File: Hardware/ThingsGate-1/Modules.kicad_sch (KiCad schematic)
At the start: 5 parts, among them SW1 DSHP03TS-S, U1 CH334R, U2 ThingsCore-1, U7 mPCIE-52P-SLOT, U8 mPCIE-52P-SLOT

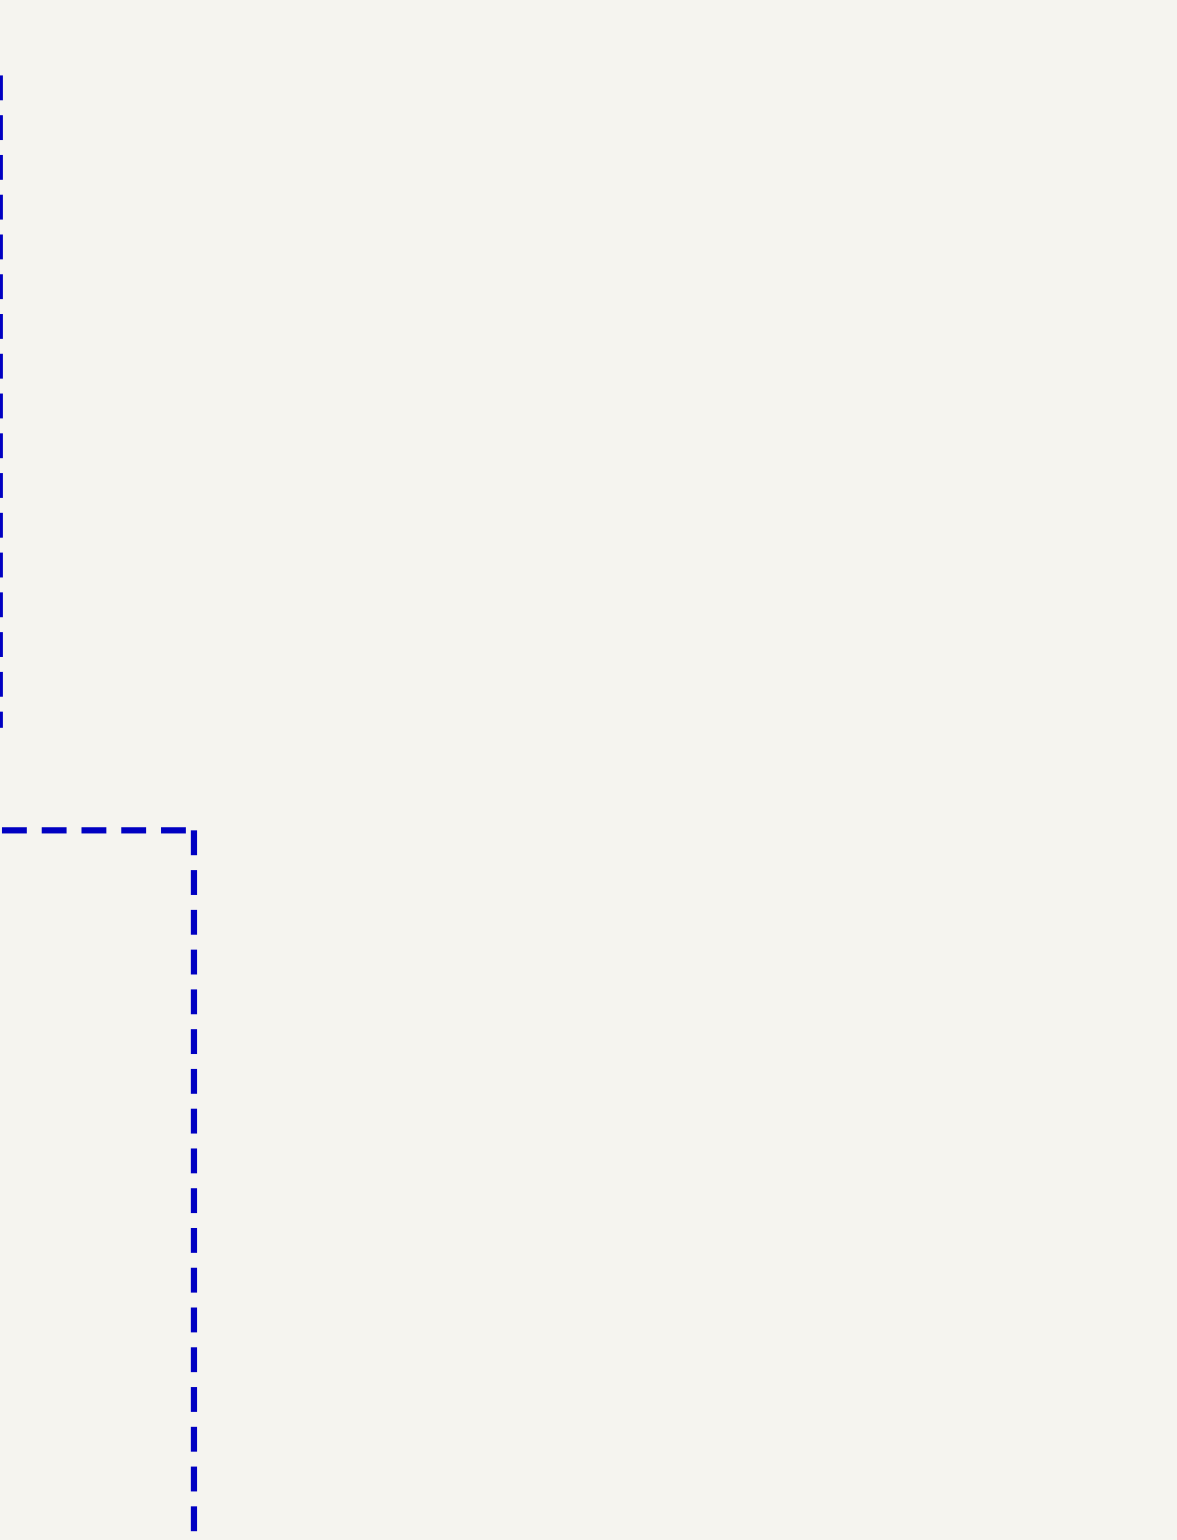
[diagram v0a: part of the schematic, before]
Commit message: schematic
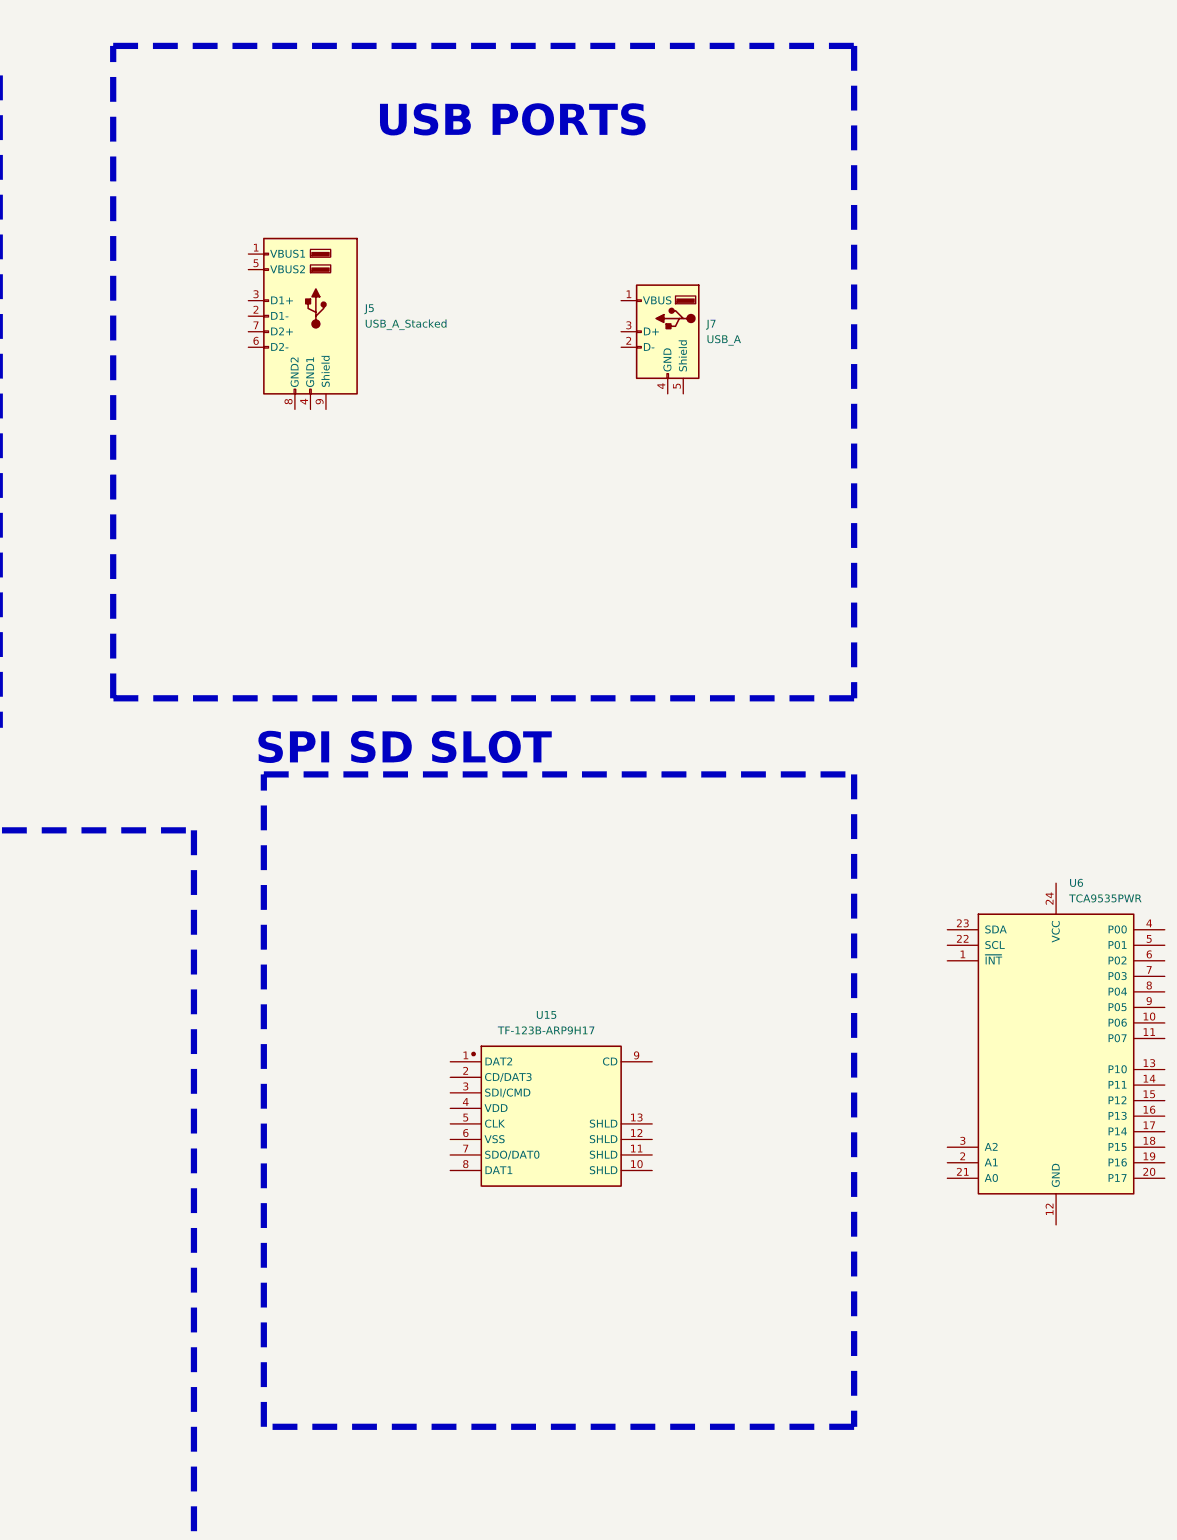
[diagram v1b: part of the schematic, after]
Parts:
- added J5: USB_A_Stacked, ThingsGate-1:DUAL_USB-TYPE_A, symbol ThingsGate-1:USB_A_Stacked
- added J7: USB_A, ThingsGate-1:USB_TYPE_A, symbol ThingsGate-1:USB_A
- added U15: TF-123B-ARP9H17, ThingsGate-1:TF-SMD_TF-123-ARP9H15, symbol ThingsGate-1:TF-123B-ARP9H17
- added U6: TCA9535PWR, Package_SO:SSOP-24_5.3x8.2mm_P0.65mm, symbol Interface_Expansion:TCA9535PWR
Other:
- note added: "SPI SD SLOT"
- note added: "USB PORTS"

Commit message: harvester schematic ready
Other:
- note added: "GPIO EXPANDER"
- moved on the sheet: U6, U7, U8
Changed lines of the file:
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@@
 	(rectangle
 		(start 21.844 149.098)
-		(end 160.02 268.478)
+		(end 116.84 268.478)
 		(stroke
 			(width 1.016)
@@
 	)
 	(rectangle
-		(start 168.402 148.844)
-		(end 290.83 267.97)
+		(start 130.302 148.844)
+		(end 200.66 267.97)
 		(stroke
 			(width 1.016)
@@
 	)
 	(rectangle
+		(start 209.55 149.86)
+		(end 294.64 267.97)
+		(stroke
+			(width 1.016)
+			(type dash)
+			(color 132 0 0 1)
+		)
+		(fill
+			(type none)
+		)
+	)
+	(rectangle
 		(start 302.26 139.7)
 		(end 398.78 246.38)
@@
 		(fill
 			(type none)
+		)
+	)
+	(text "GPIO EXPANDER\n"
+		(exclude_from_sim no)
+		(at 237.236 145.288 0)
+		(effects
+			(font
+				(size 5.08 5.08)
+				(thickness 1.016)
+				(bold yes)
+				(color 0 0 255 1)
+			)
 		)
 	)
@@
 	(text "LORAWAN GW SOM"
 		(exclude_from_sim no)
-		(at 202.692 145.034 0)
+		(at 164.592 145.034 0)
 		(effects
 			(font
@@
 	(symbol
 		(lib_id "ThingsGate-1:mPCIE-52P-SLOT")
-		(at 85.09 243.84 0)
+		(at 64.77 245.11 0)
 		(unit 1)
 		(exclude_from_sim no)
@@
 		(fields_autoplaced yes)
 		(property "Reference" "U7"
-			(at 85.09 168.91 0)
+			(at 64.77 170.18 0)
 			(effects
 				(font
@@
 		)
 		(property "Value" "mPCIE-52P-SLOT"
-			(at 85.09 171.45 0)
+			(at 64.77 172.72 0)
 			(effects
 				(font
@@
 		)
 		(property "Footprint" "ThingsGate-1:mpcie-slot_full"
-			(at 86.36 250.698 0)
+			(at 66.04 251.968 0)
 			(effects
 				(font
@@
 		)
 		(property "Datasheet" ""
-			(at 85.09 243.84 0)
+			(at 64.77 245.11 0)
 			(effects
 				(font
@@
 		)
 		(property "Description" ""
-			(at 85.09 243.84 0)
+			(at 64.77 245.11 0)
 			(effects
 				(font
@@
 	(symbol
 		(lib_id "Interface_Expansion:TCA9535PWR")
-		(at 431.8 185.42 0)
+		(at 251.46 200.66 0)
 		(unit 1)
 		(exclude_from_sim no)
@@
 		(fields_autoplaced yes)
 		(property "Reference" "U6"
-			(at 433.9433 157.48 0)
+			(at 253.6033 172.72 0)
 			(effects
 				(font
@@
 		)
 		(property "Value" "TCA9535PWR"
-			(at 433.9433 160.02 0)
+			(at 253.6033 175.26 0)
 			(effects
 				(font
@@
 		)
 		(property "Footprint" "Package_SO:SSOP-24_5.3x8.2mm_P0.65mm"
-			(at 458.47 210.82 0)
+			(at 278.13 226.06 0)
 			(effects
 				(font
@@
 		)
 		(property "Datasheet" "http://www.ti.com/lit/ds/symlink/tca9535.pdf"
-			(at 419.1 162.56 0)
+			(at 238.76 177.8 0)
 			(effects
 				(font
@@
 		)
 		(property "Description" "16-bit I/O expander, I2C and SMBus interface, interrupts, w/o pull-ups, TSSOP-24 package"
-			(at 431.8 185.42 0)
+			(at 251.46 200.66 0)
 			(effects
 				(font
@@
 	(symbol
 		(lib_id "ThingsGate-1:mPCIE-52P-SLOT")
-		(at 220.98 242.57 0)
+		(at 163.83 242.57 0)
 		(unit 1)
 		(exclude_from_sim no)
@@
 		(fields_autoplaced yes)
 		(property "Reference" "U8"
-			(at 220.98 167.64 0)
+			(at 163.83 167.64 0)
 			(effects
 				(font
@@
 		)
 		(property "Value" "mPCIE-52P-SLOT"
-			(at 220.98 170.18 0)
+			(at 163.83 170.18 0)
 			(effects
 				(font
@@
 		)
 		(property "Footprint" "ThingsGate-1:mpcie-slot_full"
-			(at 222.25 249.428 0)
+			(at 165.1 249.428 0)
 			(effects
 				(font
@@
 		)
 		(property "Datasheet" ""
-			(at 220.98 242.57 0)
+			(at 163.83 242.57 0)
 			(effects
 				(font
@@
 		)
 		(property "Description" ""
-			(at 220.98 242.57 0)
-			(effects
-				(font
+			(at 163.83 242.57 0)
+			(effects
+				(font
